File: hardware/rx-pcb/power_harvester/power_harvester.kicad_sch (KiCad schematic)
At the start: 47 parts, among them J1 Conn_Coaxial_Small, J2 Conn_01x02_Pin, J3 Conn_Coaxial_Small, J4 Conn_Coaxial_Small

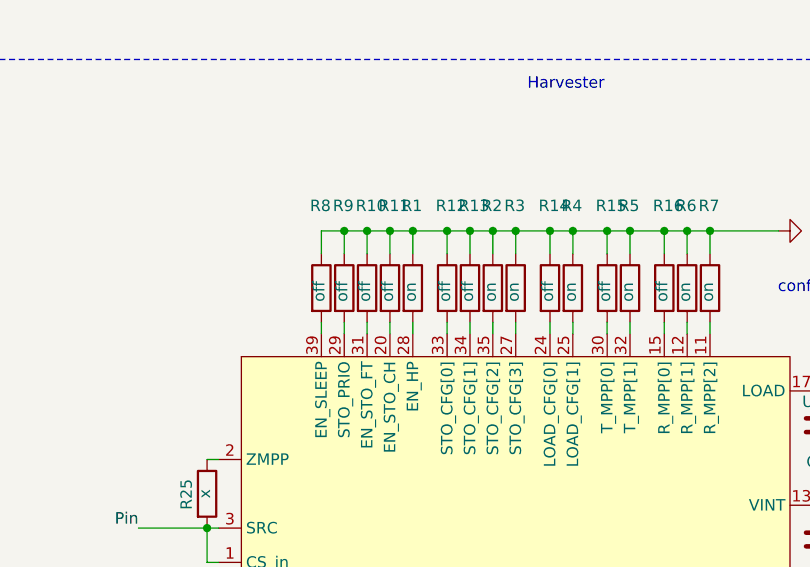
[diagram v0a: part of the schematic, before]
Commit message: updates for dr weeks
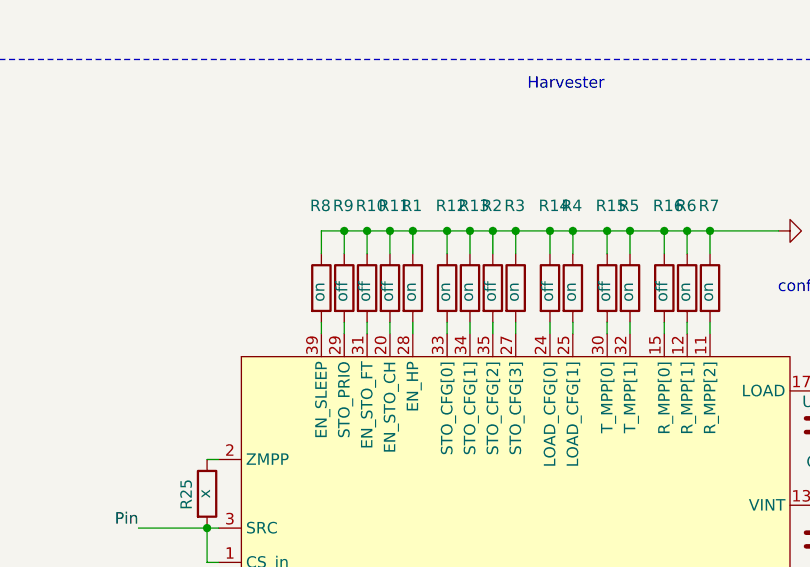
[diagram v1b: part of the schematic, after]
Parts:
- C8: footprint (none) -> Capacitor_SMD:C_0805_2012Metric_Pad1.18x1.45mm_HandSolder
- J3, J4: footprint Connector_PinHeader_2.54mm:PinHeader_1x02_P2.54mm_Vertical -> Connector_Coaxial:SMA_Molex_73251-2120_EdgeMount_Horizontal
- L1, L3: footprint Inductor_SMD:L_0805_2012Metric_Pad1.05x1.20mm_HandSolder -> Inductor_SMD:L_0402_1005Metric
- R12, R13, R8: value off -> on
- R2: value on -> off
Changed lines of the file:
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@@
 			)
 		)
-		(property "Footprint" "Inductor_SMD:L_0805_2012Metric_Pad1.05x1.20mm_HandSolder"
+		(property "Footprint" "Inductor_SMD:L_0402_1005Metric"
 			(at 58.42 43.18 0)
 			(hide yes)
@@
 			)
 		)
-		(property "Value" "off"
+		(property "Value" "on"
 			(at 49.276 120.904 90)
 			(show_name no)
@@
 			)
 		)
-		(property "Footprint" ""
+		(property "Footprint" "Capacitor_SMD:C_0805_2012Metric_Pad1.18x1.45mm_HandSolder"
 			(at 164.1348 49.53 0)
 			(hide yes)
@@
 			)
 		)
-		(property "Footprint" "Inductor_SMD:L_0805_2012Metric_Pad1.05x1.20mm_HandSolder"
+		(property "Footprint" "Inductor_SMD:L_0402_1005Metric"
 			(at 58.42 48.26 0)
 			(hide yes)
@@
 			)
 		)
-		(property "Value" "off"
+		(property "Value" "on"
 			(at 63.246 120.904 90)
 			(show_name no)
@@
 			)
 		)
-		(property "Value" "on"
+		(property "Value" "off"
 			(at 68.326 120.904 90)
 			(show_name no)
@@
 			)
 		)
-		(property "Footprint" "Connector_PinHeader_2.54mm:PinHeader_1x02_P2.54mm_Vertical"
+		(property "Footprint" "Connector_Coaxial:SMA_Molex_73251-2120_EdgeMount_Horizontal"
 			(at 184.15 33.02 0)
 			(hide yes)
@@
 			)
 		)
-		(property "Footprint" "Connector_PinHeader_2.54mm:PinHeader_1x02_P2.54mm_Vertical"
+		(property "Footprint" "Connector_Coaxial:SMA_Molex_73251-2120_EdgeMount_Horizontal"
 			(at 123.19 33.02 0)
 			(hide yes)
@@
 			)
 		)
-		(property "Value" "off"
+		(property "Value" "on"
 			(at 65.786 120.904 90)
 			(show_name no)
